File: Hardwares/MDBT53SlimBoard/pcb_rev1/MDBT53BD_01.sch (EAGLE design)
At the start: 6 parts, among them U1 RV-3028-C7

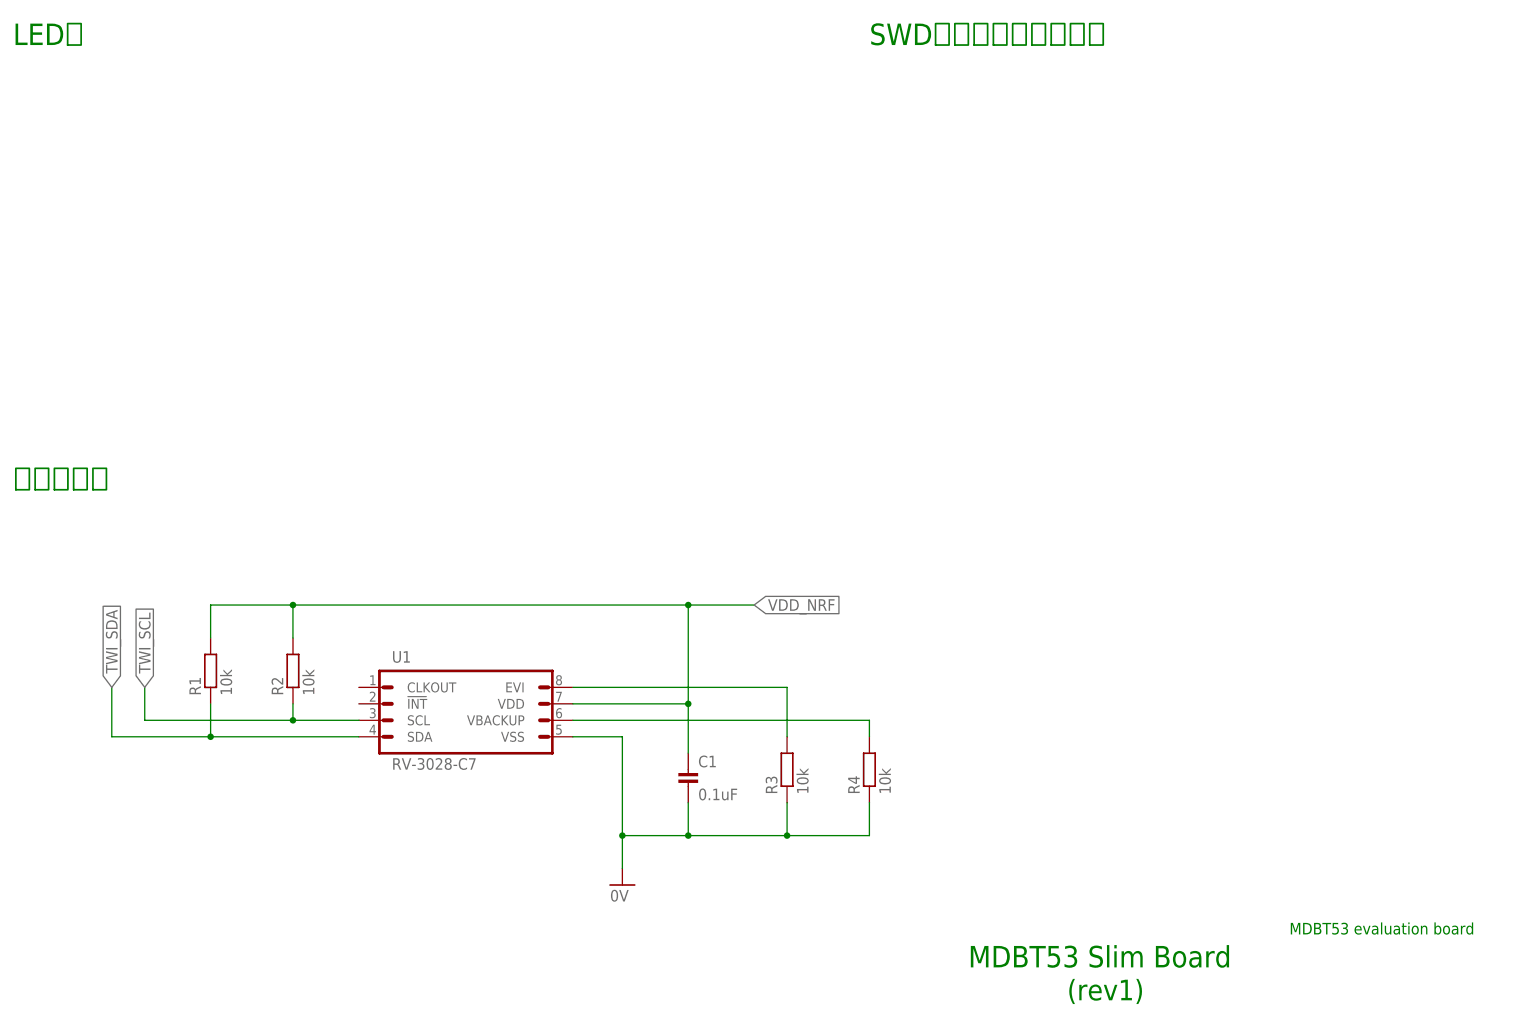
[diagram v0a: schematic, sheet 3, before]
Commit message: 回路図の作成
・LED部、SWD I/F部を追加
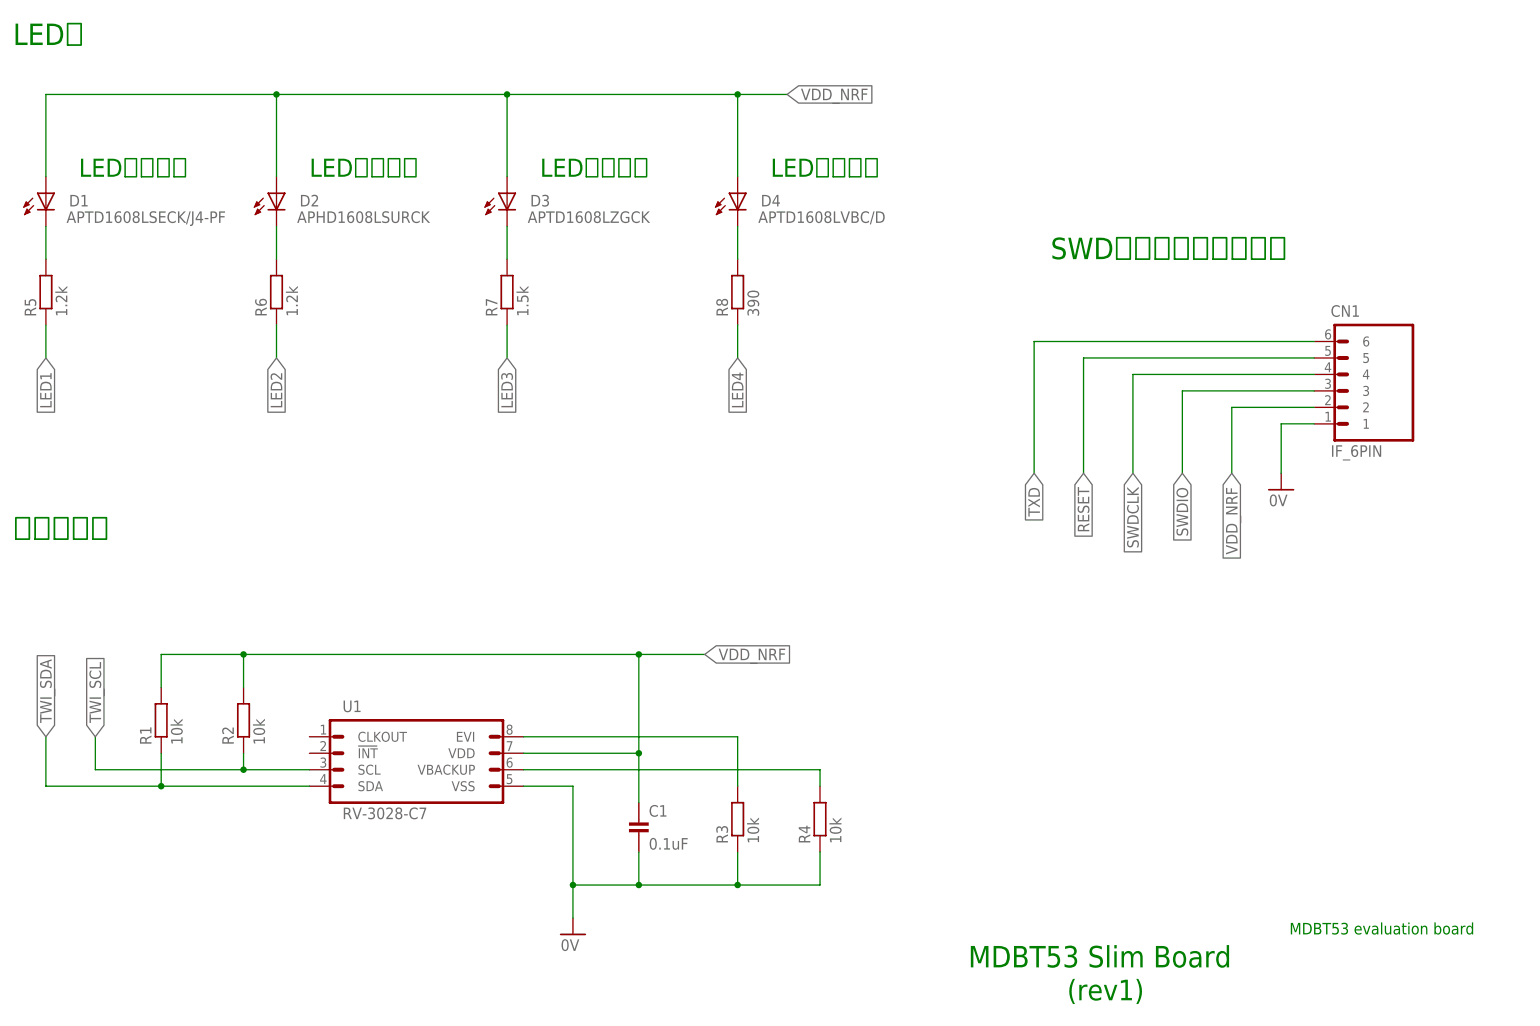
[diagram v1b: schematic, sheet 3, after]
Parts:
- added CN1: IF_6PIN, Connectors:IF_6PIN
- added D1: APTD1608LSECK/J4-PF, Parts:APTD1608LSECK/J4-PF
- added D2: APHD1608LSURCK, Parts:APHD1608LSURCK
- added D3: APTD1608LZGCK, Parts:APTD1608LZGCK
- added D4: APTD1608LVBC/D, Parts:APTD1608LVBC/D
- added R5, R6: 1.2k, Parts:RESISTOR_0402N
- added R7: 1.5k, Parts:RESISTOR_0402N
- added R8: 390, Parts:RESISTOR_0402N
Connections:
- new net LED1: R5.1
- new net LED2: R6.1
- new net LED3: R7.1
- new net LED4: R8.1
- new net N$1: D1.C, R5.2
- new net N$4: D2.C, R6.2
- new net N$5: D3.C, R7.2
- new net N$6: D4.C, R8.2
- new net RESET: CN1.5
- new net SWDCLK: CN1.4
- new net SWDIO: CN1.3
- new net TXD: CN1.6
- net 0V: now also CN1.1
- net VDD_NRF: now also CN1.2, D1.A, D2.A, D3.A, D4.A
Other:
- note added: "LED（緑色）"
- note added: "LED（赤色）"
- note added: "LED（青色）"
- note added: "LED（黄色）"
- moved on the sheet: C1, R1, R2, R3, R4, U1
